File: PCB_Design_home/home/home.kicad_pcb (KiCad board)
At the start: 2 copper layers, 48.2 x 62.3 mm, 54 parts, among them J1 10155435-00011LF, J2 Conn_01x05_Socket, J3 Conn_01x04_Socket, Q1 2N3904, Q2 2N3904, SW1 1825910-6, SW2 1825910-6, SW4 1825910-6, U1 ESP32-C3-WROOM-02, U2 CP2102N-Axx-xQFN28, U3 ULN2003A, U4 BME680, U5 AMS1117-3.3

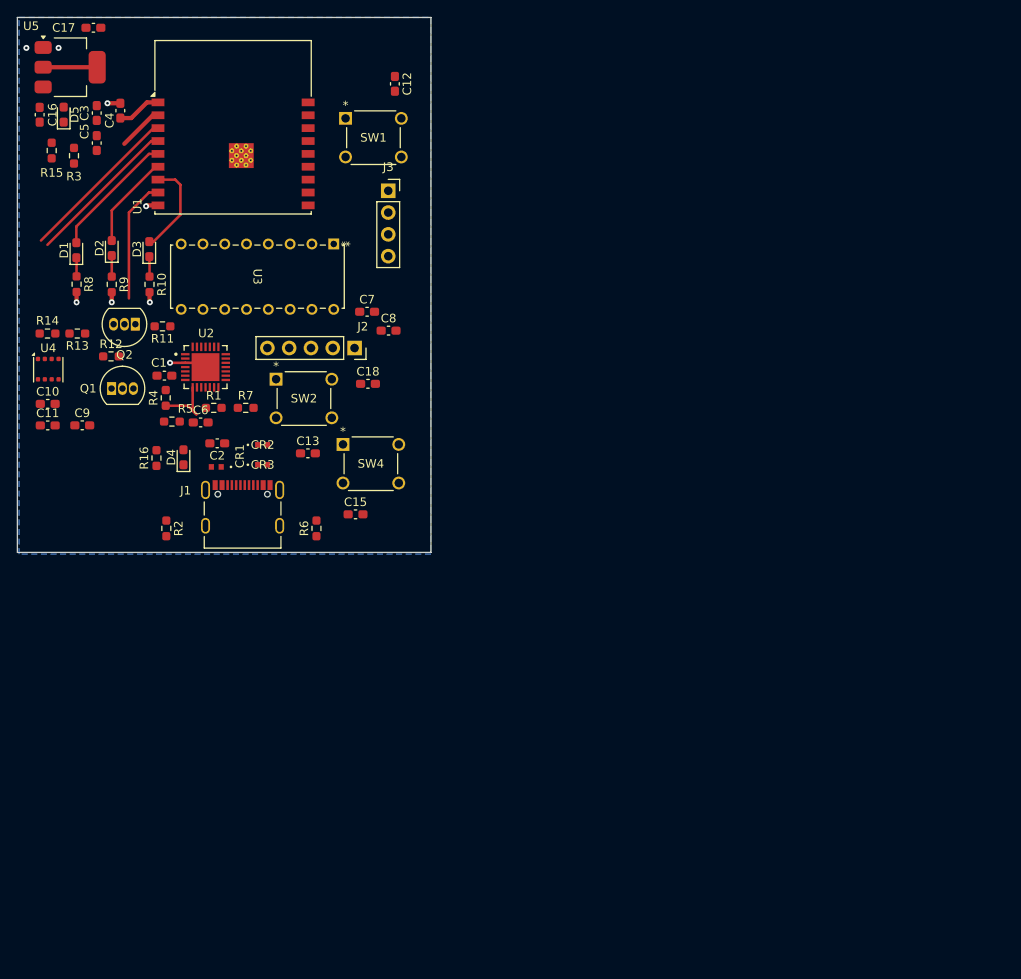
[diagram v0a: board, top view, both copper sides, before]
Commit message: Update
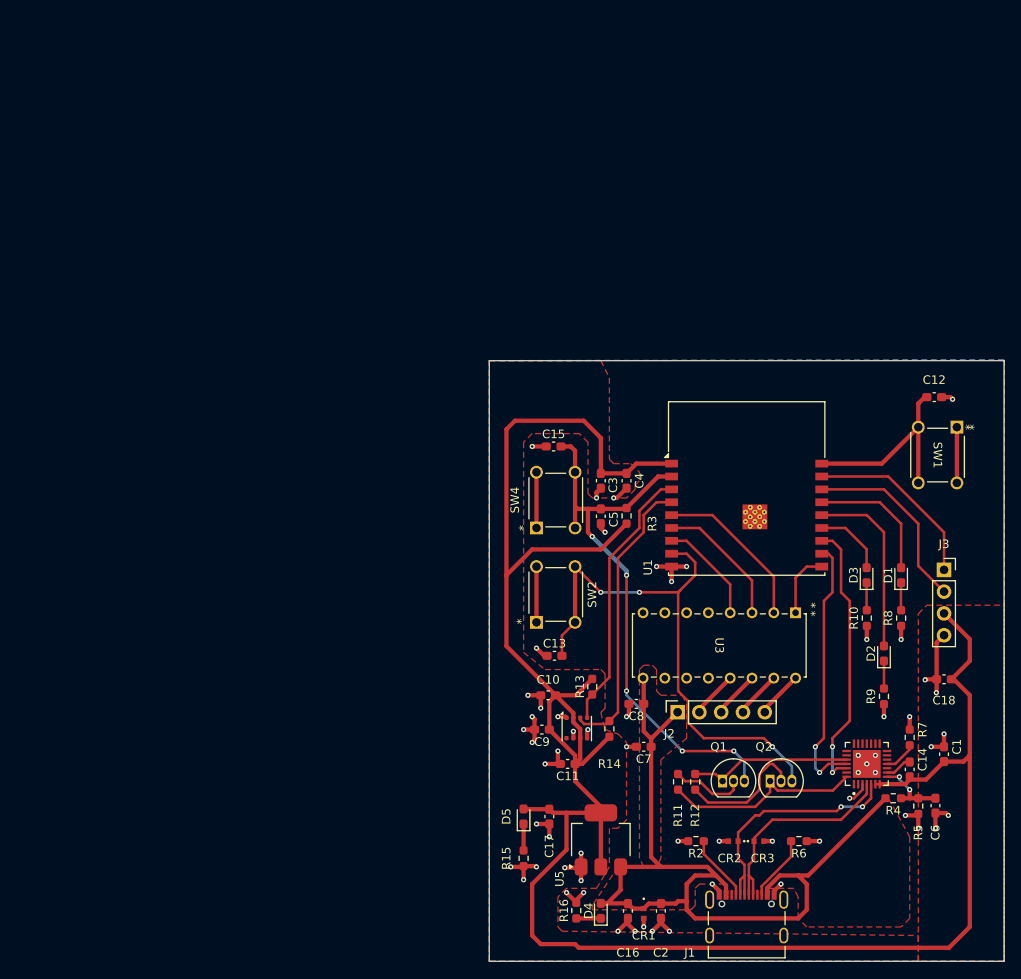
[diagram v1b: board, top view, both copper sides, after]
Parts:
- removed R1: 1k, Resistor_SMD:R_0603_1608Metric_Pad0.98x0.95mm_HandSolder
- added C14: 4.7uF, Capacitor_SMD:C_0603_1608Metric_Pad1.08x0.95mm_HandSolder, F.Cu at (229.0, 137.6)
- C1: value 10uF -> 0.1uF
- moved C16 115.4 mm to (196.2, 154.1), turned to -90 degrees
- moved U5 109.2 mm to (193.0, 145.8), turned to 90 degrees
- moved C17 106.2 mm to (187.0, 143.1), turned to -90 degrees
- moved R8 103.7 mm to (228.0, 120.0)
- moved D1 103.3 mm to (228.0, 115.0)
- moved R9 102.0 mm to (226.0, 129.1)
- moved D2 101.6 mm to (226.0, 124.1)
- moved C1 101.0 mm to (233.0, 135.9), turned to 90 degrees
- moved R15 99.1 mm to (184.0, 148.0)
- moved R5 97.9 mm to (230.0, 141.9), turned to 90 degrees
- moved D5 97.8 mm to (184.0, 143.1)
- moved R4 96.8 mm to (227.1, 141.0), turned to 180 degrees
- moved C6 96.6 mm to (232.0, 141.9), turned to -90 degrees
- moved R10 92.2 mm to (224.0, 120.0)
- moved D3 91.8 mm to (224.0, 115.0)
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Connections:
- C18 pad 1: +5V -> +3.3V
- J3 pad 3: +5V -> +3.3V
- U1 pad 11: /motor2 -> /RXD
- U1 pad 12: /motor3 -> /TXD
- U1 pad 13: /motor4 -> Net-(D3-A)
- U1 pad 14: /TXD -> Net-(D2-A)
- U1 pad 15: /RXD -> Net-(D1-A)
- U1 pad 5: Net-(D1-A) -> /motor2
- U1 pad 6: Net-(D2-A) -> /motor3
- U1 pad 7: Net-(D3-A) -> /motor4
- U3 pad 13: Net-(J2-Pin_5) -> Net-(J2-Pin_2)
- U3 pad 14: Net-(J2-Pin_4) -> Net-(J2-Pin_3)
- U3 pad 15: Net-(J2-Pin_3) -> Net-(J2-Pin_4)
- U3 pad 16: Net-(J2-Pin_2) -> Net-(J2-Pin_5)
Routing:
- net +3.3V: track 11.4 -> 247.4 mm
- net +5V: track 0.00 -> 103.1 mm
- net GND: track 10.9 -> 109.2 mm, vias 8 -> 60
- net /EN: track 5.30 -> 66.6 mm, vias 0 -> 5
- net /IO9: track 14.4 -> 63.7 mm, vias 0 -> 3
- net /TXD: track 0.00 -> 31.8 mm, vias 0 -> 2
- net /RXD: track 0.40 -> 31.0 mm, vias 0 -> 2
- net /USB_D-: track 0.00 -> 28.8 mm, vias 0 -> 2
- net /USB_D+: track 0.00 -> 25.7 mm
- net /DTR: track 0.00 -> 23.7 mm
- net /Tastknopf1: track 0.00 -> 23.6 mm
- net /SDA_display: track 0.00 -> 22.1 mm
- net /SCK_display: track 0.00 -> 21.3 mm
- net /RTS: track 0.00 -> 19.1 mm
- net /motor2: track 0.00 -> 19.1 mm
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- added copper zone on F.Cu, net +3.3V
- added copper zone on F.Cu, net +5V
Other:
- board size 48.2 x 62.3 mm -> 60 x 70 mm
